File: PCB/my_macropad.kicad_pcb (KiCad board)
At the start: 2 copper layers, 58 x 50 mm, 8 parts, among them SW1 SW_Push, SW2 SW_Push, SW3 SW_Push, SW4 SW_Push, U1 MOUDLE-SEEEDUINO-XIAO, U2 ER_OLEDM0.91_1x-I2C

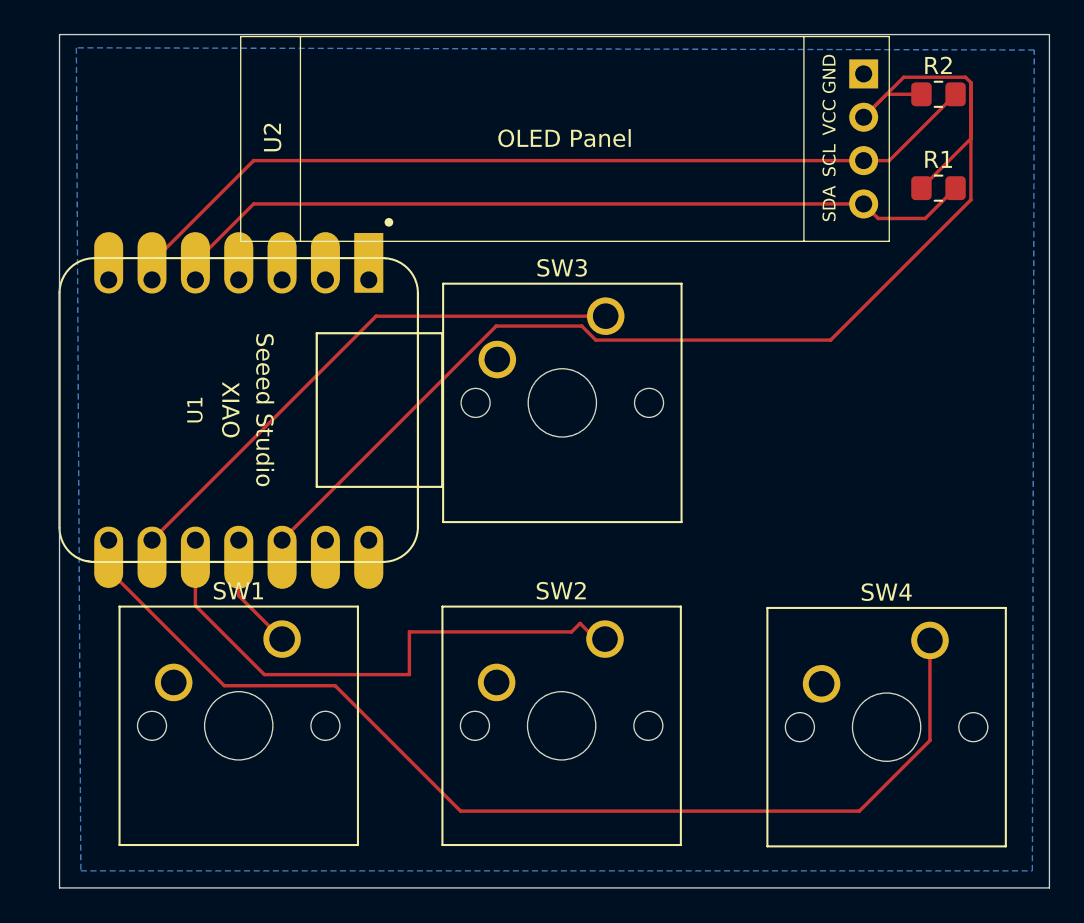
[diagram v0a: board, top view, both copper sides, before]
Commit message: fixed changes asked
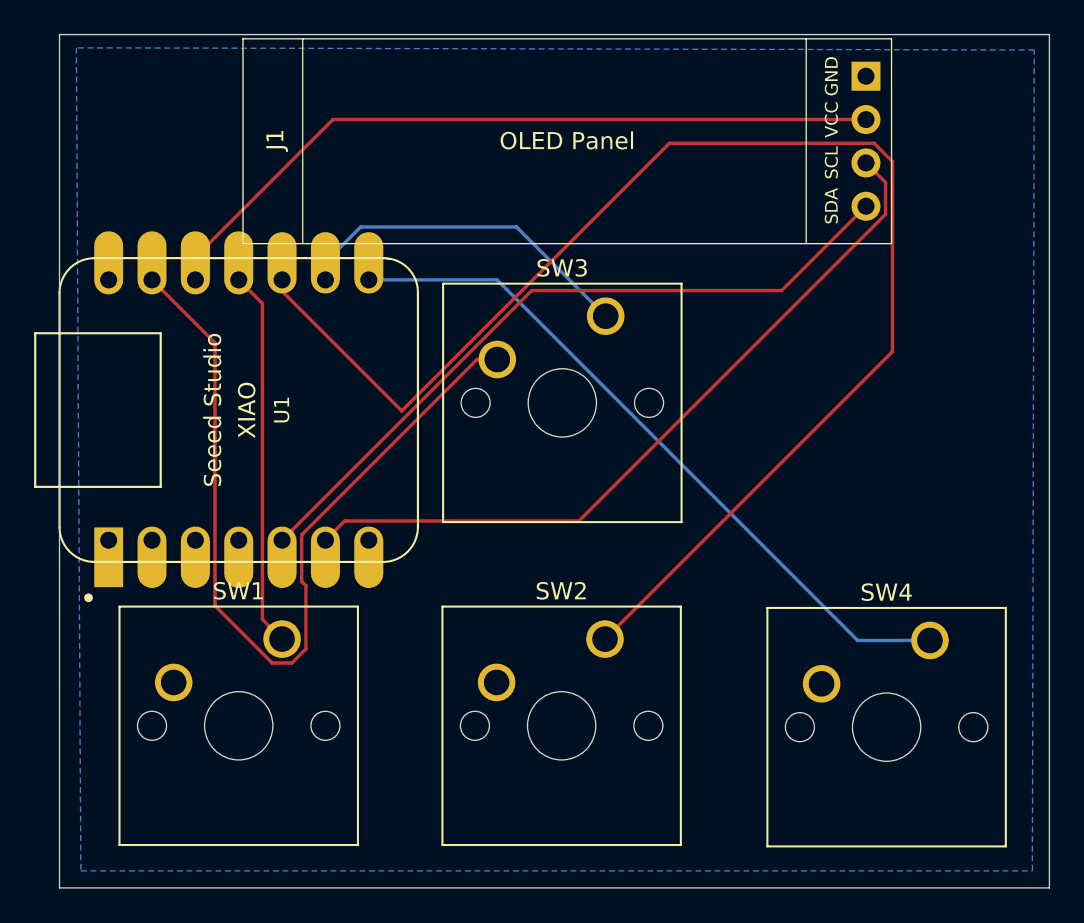
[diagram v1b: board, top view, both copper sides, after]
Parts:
- removed R1, R2: R, Resistor_SMD:R_0805_2012Metric_Pad1.20x1.40mm_HandSolder
- removed U2: ER_OLEDM0.91_1x-I2C, KiCad-SSD1306-0.91-OLED-4pin-128x32:SSD1306-0.91-OLED-4pin-128x32
- added J1: Conn_01x04, KiCad-SSD1306-0.91-OLED-4pin-128x32:SSD1306-0.91-OLED-4pin-128x32, F.Cu at (89.8, 74.2)
- turned U1 to 90 degrees
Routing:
- net GND: track 0.00 -> 50.2 mm
- net Net-(U1-PA5_A9_D9_MISO): track 32.6 -> 81.2 mm
- net VCC: track 74.9 -> 44.0 mm
- net Net-(U1-PB09_A7_D7_RX): track 63.3 -> 41.6 mm
- net Net-(U1-PA6_A10_D10_MOSI): track 6.85 -> 22.1 mm
- net Net-(U1-PA7_A8_D8_SCK): track 32.0 -> 20.5 mm
- net Net-(J1-Pin_3): track 52.2 -> 44.2 mm
- net Net-(J1-Pin_4): track 48.1 -> 42.3 mm
